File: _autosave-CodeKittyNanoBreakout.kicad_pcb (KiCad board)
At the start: 2 copper layers, 17.8 x 43.2 mm, 14 parts, among them P1 CONN_01X02, P2 CONN_01X02, P3 CONN_01X03, P4 CONN_01X03, P5 CONN_01X02, SW1 SW_PUSH_SMALL_H, SW2 Switch_SPDT_x2, U1 ArduinoNano

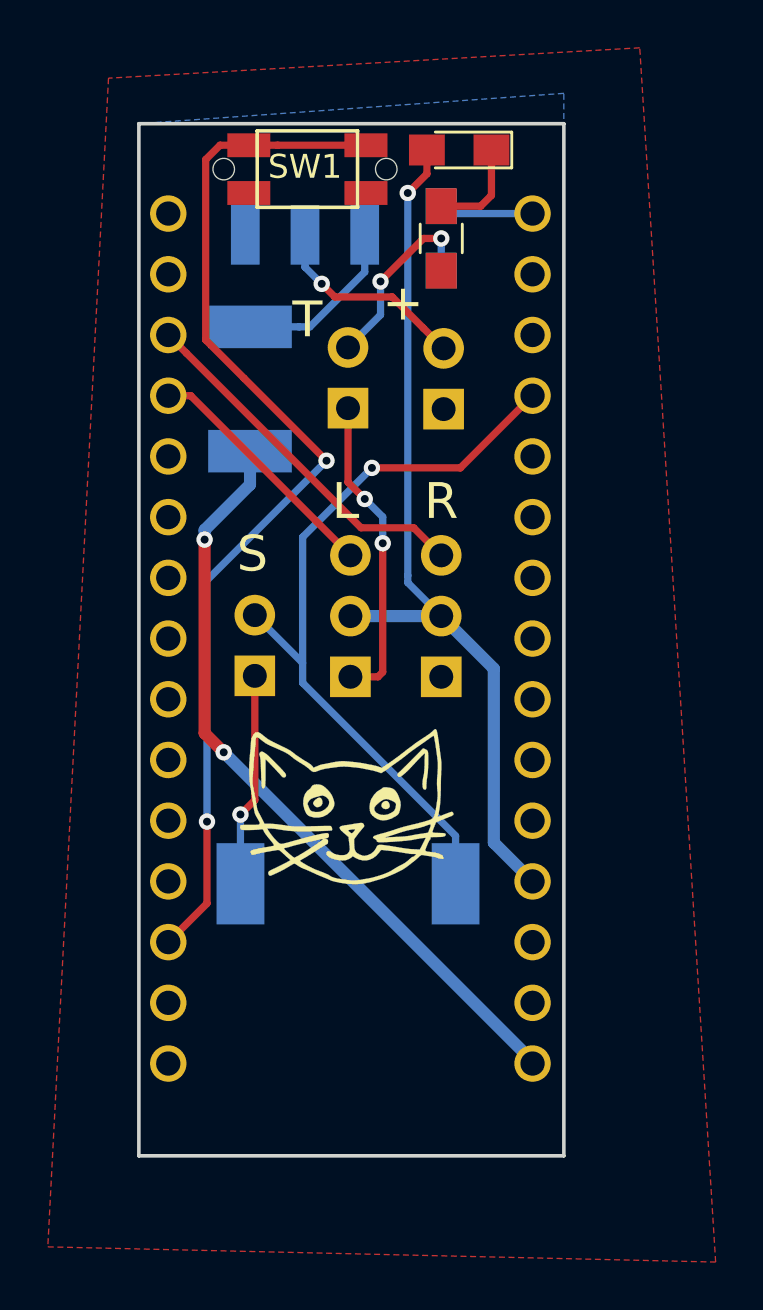
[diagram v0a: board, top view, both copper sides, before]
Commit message: ...
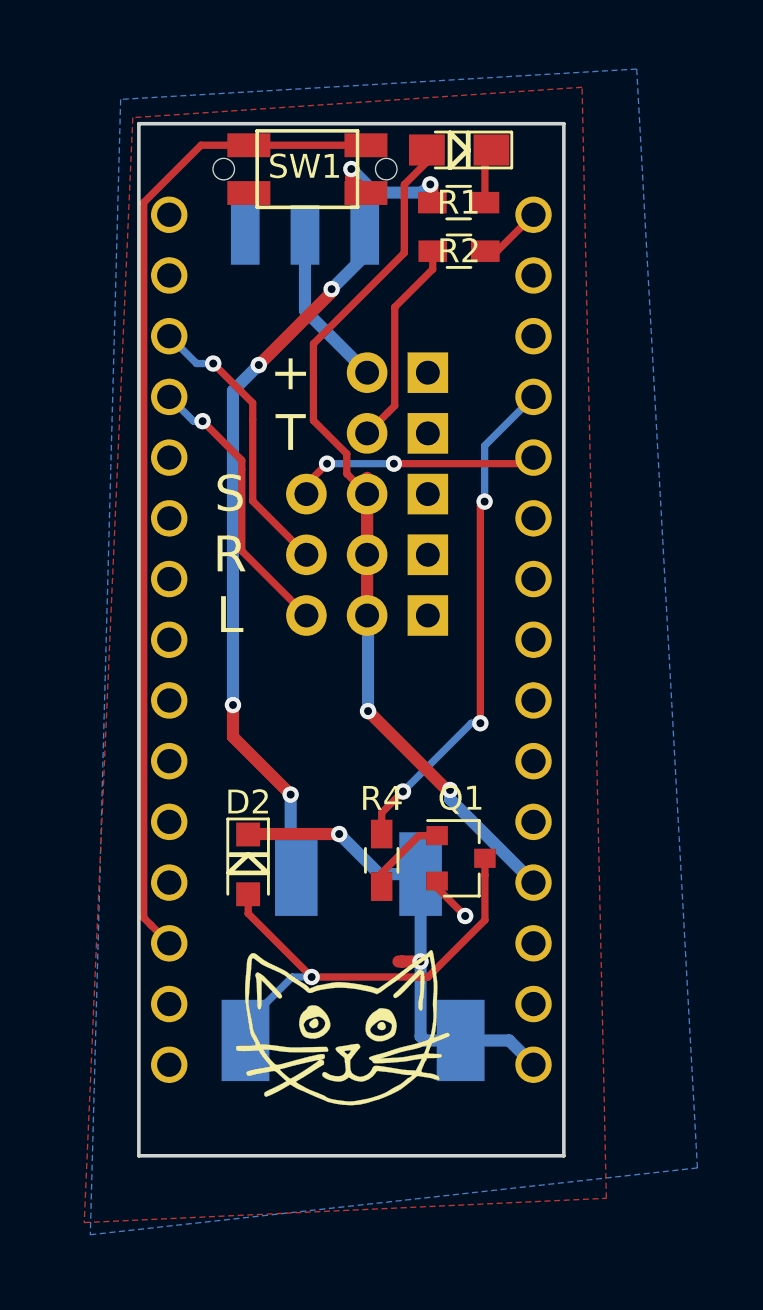
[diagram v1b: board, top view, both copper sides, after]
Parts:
- added D2: D, Diodes_SMD:D_SOD-323_HandSoldering, F.Cu at (201.4, 113.5)
- added Q1: MMBT3904, TO_SOT_Packages_SMD:SOT-23, F.Cu at (210.3, 113.3)
- added R4: 1K, Resistors_SMD:R_0603_HandSoldering, F.Cu at (207.0, 113.4)
- P5: value CONN_01X02 -> CONN_01X03; footprint Pin_Headers:Pin_Header_Straight_1x02_Pitch2.54mm -> Pin_Headers:Pin_Header_Straight_1x03_Pitch2.54mm
- R1: footprint Resistors_SMD:R_0805_HandSoldering -> Resistors_SMD:R_0603_HandSoldering
- R2: footprint Resistors_SMD:R_0805_HandSoldering -> Resistors_SMD:R_0603_HandSoldering; moved to F.Cu
- SP1: value SPEAKER -> PIEZO
- moved F1 20.8 mm to (206.0, 113.9), turned to 180 degrees
- moved P5 10.5 mm to (208.9, 98.0), turned to 90 degrees
- moved G*** 9.25 mm to (205.2, 120.4)
- moved SP1 6.56 mm to (205.8, 120.9)
- moved P4 5.13 mm to (208.9, 100.6), turned to 90 degrees
- moved P3 4.13 mm to (208.9, 103.1), turned to 90 degrees
- moved P2 3.50 mm to (208.9, 95.5), turned to 90 degrees
- moved R1 1.67 mm to (210.2, 85.9), turned to 180 degrees
- moved P1 1.66 mm to (208.9, 93.0), turned to 90 degrees
- moved R2 0.92 mm to (210.2, 87.9), turned to 0 degrees
- moved U1 0.06 mm to (205.7, 104.1)
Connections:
- P5 pad 2: BUZZ -> 5V
- SP1 pad 1: BUZZ -> VCC
- SP1 pad 2: GND -> Net-(D2-Pad2)
- U1 pad 20: Net-(U1-Pad20) -> SENS
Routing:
- net Net-(F1-Pad1): track 7.31 -> 31.6 mm, vias 0 -> 4
- net Net-(D2-Pad2): track 0.00 -> 19.7 mm, vias 0 -> 1
- net GND: track 22.0 -> 7.86 mm
- net VCC: track 32.1 -> 20.9 mm
- net BUZZ: track 32.1 -> 21.1 mm, vias 1 -> 3
- net SENS: track 0.00 -> 10.4 mm, vias 0 -> 2
- net Net-(Q1-Pad1): track 0.00 -> 3.54 mm
- net RSERVO: track 15.2 -> 11.9 mm, vias 0 -> 1
- net RST: track 44.5 -> 41.7 mm, vias 2 -> 0
- net Net-(D1-Pad1): track 4.19 -> 2.31 mm
- net Net-(P1-Pad2): track 8.56 -> 6.84 mm, vias 1 -> 0
- net LSERVO: track 10.4 -> 11.7 mm, vias 0 -> 1
- net TAIL: track 3.95 -> 2.65 mm
- net 5V: track 36.8 -> 37.2 mm, vias 1 -> 2
- net Net-(P2-Pad2): track 8.66 -> 8.76 mm, vias 2 -> 0
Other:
- board text added: "CodeKitty v1.0 DM120317"
- board text removed: "CodeKitty DM100917"
